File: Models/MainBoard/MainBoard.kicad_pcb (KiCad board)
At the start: 4 copper layers, 82 parts, among them J1 Conn_Coaxial, J10 Conn_01x03_Pin, J11 Conn_01x03_Pin, J12 Conn_01x03_Pin, J13 Conn_01x02_Pin, J14 Conn_01x13_Pin, J15 Conn_01x13_Pin, J16 Conn_01x24_Socket, J19 Conn_01x24_Socket, J2 Conn_Coaxial, J3 Conn_Coaxial, J4 Conn_Coaxial, J5 Conn_Coaxial, J6 Conn_Coaxial, J7 Conn_01x03_Pin, J8 Conn_01x03_Pin, J9 Conn_01x03_Pin, U1 ADS8699, U2 AD7745, U3 DAC81404, U4 DAC81401, U5 ISO7761DW, U6 ISO1641DW

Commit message: Save progress
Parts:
- J10, J11, J12, J7, J8, J9: footprint Connector_Custom:PinConnector_1x3 -> Connector_Custom:PinHeader_1x3
- J13: footprint Connector_Custom:PinConnector_1x2 -> Connector_Custom:PinHeader_1x2
- J14, J15: footprint Connector_Custom:PinConnector_1x13 -> Connector_Custom:PinHeader_1x13
- J16, J19: footprint Connector_Custom:PinConnector_1x24 -> Connector_Custom:PinSocket_1x24
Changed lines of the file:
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@@
 		(embedded_fonts no)
 	)
-	(footprint "Connector_Custom:PinConnector_1x3"
+	(footprint "Connector_Custom:PinHeader_1x3"
 		(layer "F.Cu")
 		(at 111.86 94.16)
@@
 		)
 		(embedded_fonts no)
+		(model "${KICAD9_3DMODEL_DIR}/Connector_PinHeader_2.54mm.3dshapes/PinHeader_1x03_P2.54mm_Vertical.step"
+			(offset
+				(xyz 0 2.54 0)
+			)
+			(scale
+				(xyz 1 1 1)
+			)
+			(rotate
+				(xyz -0 -0 -0)
+			)
+		)
 	)
 	(footprint "TwoTerminal:CAPC0805"
@@
 		(embedded_fonts no)
 	)
-	(footprint "Connector_Custom:PinConnector_1x3"
+	(footprint "Connector_Custom:PinHeader_1x3"
 		(layer "F.Cu")
 		(at 111.86 114.48)
@@
 		)
 		(embedded_fonts no)
+		(model "${KICAD9_3DMODEL_DIR}/Connector_PinHeader_2.54mm.3dshapes/PinHeader_1x03_P2.54mm_Vertical.step"
+			(offset
+				(xyz 0 2.54 0)
+			)
+			(scale
+				(xyz 1 1 1)
+			)
+			(rotate
+				(xyz -0 -0 -0)
+			)
+		)
 	)
 	(footprint "TwoTerminal:CAPC0603"
@@
 		)
 		(embedded_fonts no)
+		(model "${KIPRJMOD}/../libraries/IC.pretty/VQFN-32.step"
+			(offset
+				(xyz 0 0 0)
+			)
+			(scale
+				(xyz 1 1 1)
+			)
+			(rotate
+				(xyz -0 -0 -0)
+			)
+		)
 	)
 	(footprint "Connector_Custom:NetTie_0.2mm"
@@
 		(embedded_fonts no)
 	)
-	(footprint "Connector_Custom:PinConnector_1x24"
+	(footprint "Connector_Custom:PinSocket_1x24"
 		(layer "F.Cu")
 		(at 160.12 100.51)
@@
 		)
 		(embedded_fonts no)
+		(model "${KICAD9_3DMODEL_DIR}/Connector_PinSocket_2.54mm.3dshapes/PinSocket_1x24_P2.54mm_Vertical.step"
+			(offset
+				(xyz 0 29.21 0)
+			)
+			(scale
+				(xyz 1 1 1)
+			)
+			(rotate
+				(xyz -0 -0 -0)
+			)
+		)
 	)
 	(footprint "Connector_Custom:NetTie_0.2mm"
@@
 		(embedded_fonts no)
 	)
-	(footprint "Connector_Custom:PinConnector_1x24"
+	(footprint "Connector_Custom:PinSocket_1x24"
 		(layer "F.Cu")
 		(at 175.36 100.51 180)
@@
 		)
 		(embedded_fonts no)
+		(model "${KICAD9_3DMODEL_DIR}/Connector_PinSocket_2.54mm.3dshapes/PinSocket_1x24_P2.54mm_Vertical.step"
+			(offset
+				(xyz 0 29.21 0)
+			)
+			(scale
+				(xyz 1 1 1)
+			)
+			(rotate
+				(xyz -0 -0 -0)
+			)
+		)
 	)
-	(footprint "Connector_Custom:PinConnector_1x3"
+	(footprint "Connector_Custom:PinHeader_1x3"
 		(layer "F.Cu")
 		(at 111.86 124.64)
@@
 		)
 		(embedded_fonts no)
+		(model "${KICAD9_3DMODEL_DIR}/Connector_PinHeader_2.54mm.3dshapes/PinHeader_1x03_P2.54mm_Vertical.step"
+			(offset
+				(xyz 0 2.54 0)
+			)
+			(scale
+				(xyz 1 1 1)
+			)
+			(rotate
+				(xyz -0 -0 -0)
+			)
+		)
 	)
 	(footprint "TwoTerminal:CAPC0603"
@@
 		(embedded_fonts no)
 	)
-	(footprint "Connector_Custom:PinConnector_1x2"
+	(footprint "Connector_Custom:PinHeader_1x2"
 		(layer "F.Cu")
 		(at 105.51 129.72 90)
@@
 		)
 		(embedded_fonts no)
+		(model "${KICAD9_3DMODEL_DIR}/Connector_PinHeader_2.54mm.3dshapes/PinHeader_1x02_P2.54mm_Vertical.step"
+			(offset
+				(xyz 0 1.27 0)
+			)
+			(scale
+				(xyz 1 1 1)
+			)
+			(rotate
+				(xyz -0 -0 -0)
+			)
+		)
 	)
 	(footprint "TwoTerminal:CAPC0805"
@@
 		)
 		(embedded_fonts no)
+		(model "${KIPRJMOD}/../libraries/Connector_Custom.pretty/Keystone_24929.step"
+			(offset
+				(xyz 0 0 -1.5)
+			)
+			(scale
+				(xyz 1 1 1)
+			)
+			(rotate
+				(xyz -90 -0 -0)
+			)
+		)
 	)
 	(footprint "Connector_Custom:NetTie_0.2mm"
@@
 		(embedded_fonts no)
 	)
-	(footprint "Connector_Custom:PinConnector_1x3"
+	(footprint "Connector_Custom:PinHeader_1x3"
 		(layer "F.Cu")
 		(at 111.86 73.84)
@@
 		)
 		(embedded_fonts no)
+		(model "${KICAD9_3DMODEL_DIR}/Connector_PinHeader_2.54mm.3dshapes/PinHeader_1x03_P2.54mm_Vertical.step"
+			(offset
+				(xyz 0 2.54 0)
+			)
+			(scale
+				(xyz 1 1 1)
+			)
+			(rotate
+				(xyz -0 -0 -0)
+			)
+		)
 	)
 	(footprint "TwoTerminal:CAPC0603"
@@
 		(embedded_fonts no)
 	)
-	(footprint "Connector_Custom:PinConnector_1x3"
+	(footprint "Connector_Custom:PinHeader_1x3"
 		(layer "F.Cu")
 		(at 111.86 104.32)
@@
 		)
 		(embedded_fonts no)
+		(model "${KICAD9_3DMODEL_DIR}/Connector_PinHeader_2.54mm.3dshapes/PinHeader_1x03_P2.54mm_Vertical.step"
+			(offset
+				(xyz 0 2.54 0)
+			)
+			(scale
+				(xyz 1 1 1)
+			)
+			(rotate
+				(xyz -0 -0 -0)
+			)
+		)
 	)
 	(footprint "TwoTerminal:CAPC0805"
@@
 		(embedded_fonts no)
 	)
-	(footprint "Connector_Custom:PinConnector_1x3"
+	(footprint "Connector_Custom:PinHeader_1x3"
 		(layer "F.Cu")
 		(at 111.86 84)
@@
 		)
 		(embedded_fonts no)
+		(model "${KICAD9_3DMODEL_DIR}/Connector_PinHeader_2.54mm.3dshapes/PinHeader_1x03_P2.54mm_Vertical.step"
+			(offset
+				(xyz 0 2.54 0)
+			)
+			(scale
+				(xyz 1 1 1)
+			)
+			(rotate
+				(xyz -0 -0 -0)
+			)
+		)
 	)
 	(footprint "TwoTerminal:CAPC0603"
@@
 		)
 		(embedded_fonts no)
+		(model "${KIPRJMOD}/../libraries/Connector_Custom.pretty/Molex_MCX.step"
+			(offset
+				(xyz -6.53 0 3.3)
+			)
+			(scale
+				(xyz 1 1 1)
+			)
+			(rotate
+				(xyz -90 -0 90)
+			)
+		)
 	)
 	(footprint "TwoTerminal:RESC0603"
@@
 		)
 		(embedded_fonts no)
+		(model "${KIPRJMOD}/../libraries/Connector_Custom.pretty/Molex_MCX.step"
+			(offset
+				(xyz -6.53 0 3.3)
+			)
+			(scale
+				(xyz 1 1 1)
+			)
+			(rotate
+				(xyz -90 -0 90)
+			)
+		)
 	)
 	(footprint "Connector_Custom:Molex_MCX"
@@
 		)
 		(embedded_fonts no)
+		(model "${KIPRJMOD}/../libraries/Connector_Custom.pretty/Molex_MCX.step"
+			(offset
+				(xyz -6.53 0 3.3)
+			)
+			(scale
+				(xyz 1 1 1)
+			)
+			(rotate
+				(xyz -90 -0 90)
+			)
+		)
 	)
 	(footprint "TwoTerminal:RESC0603"
@@
 		(embedded_fonts no)
 	)
-	(footprint "Connector_Custom:PinConnector_1x13"
+	(footprint "Connector_Custom:PinHeader_1x13"
 		(layer "B.Cu")
 		(at 132.18 71.3 -90)
@@
 		)
 		(property "Purchase Link" "https://www.digikey.com/en/products/detail/sullins-connector-solutions/PRPC024SAAN-RC/2775230"
-			(at 0 0 90)
+			(at 0 0 270)
 			(unlocked yes)
 			(layer "B.Fab")
@@
 		)
 		(property "Cost" "$0.563"
-			(at 0 0 90)
+			(at 0 0 270)
 			(unlocked yes)
 			(layer "B.Fab")
@@
 		)
 		(embedded_fonts no)
+		(model "${KICAD9_3DMODEL_DIR}/Connector_PinHeader_2.54mm.3dshapes/PinHeader_1x13_P2.54mm_Vertical.step"
+			(offset
+				(xyz 0 15.24 0)
+			)
+			(scale
+				(xyz 1 1 1)
+			)
+			(rotate
+				(xyz -0 -0 -0)
+			)
+		)
 	)
 	(footprint "TwoTerminal:RESC0603"
@@
 		(embedded_fonts no)
 	)
-	(footprint "Connector_Custom:PinConnector_1x13"
+	(footprint "Connector_Custom:PinHeader_1x13"
 		(layer "B.Cu")
 		(at 132.18 129.72 -90)
@@
 		)
 		(embedded_fonts no)
+		(model "${KICAD9_3DMODEL_DIR}/Connector_PinHeader_2.54mm.3dshapes/PinHeader_1x13_P2.54mm_Vertical.step"
+			(offset
+				(xyz 0 15.24 0)
+			)
+			(scale
+				(xyz 1 1 1)
+			)
+			(rotate
+				(xyz -0 -0 -0)
+			)
+		)
 	)
 	(footprint "Connector_Custom:Molex_MCX"
@@
 		)
 		(embedded_fonts no)
+		(model "${KIPRJMOD}/../libraries/Connector_Custom.pretty/Molex_MCX.step"
+			(offset
+				(xyz -6.53 0 3.3)
+			)
+			(scale
+				(xyz 1 1 1)
+			)
+			(rotate
+				(xyz -90 -0 90)
+			)
+		)
 	)
 	(footprint "TwoTerminal:RESC0603"
@@
 		)
 		(embedded_fonts no)
+		(model "${KIPRJMOD}/../libraries/Connector_Custom.pretty/Molex_MCX.step"
+			(offset
+				(xyz -6.53 0 3.3)
+			)
+			(scale
+				(xyz 1 1 1)
+			)
+			(rotate
+				(xyz -90 -0 90)
+			)
+		)
 	)
 	(footprint "Connector_Custom:Molex_MCX"
@@
 		)
 		(embedded_fonts no)
+		(model "${KIPRJMOD}/../libraries/Connector_Custom.pretty/Molex_MCX.step"
+			(offset
+				(xyz -6.53 0 3.3)
+			)
+			(scale
+				(xyz 1 1 1)
+			)
+			(rotate
+				(xyz -90 -0 90)
+			)
+		)
 	)
 	(gr_text "Nanofactory Project\nPhase 0.2/I/II"

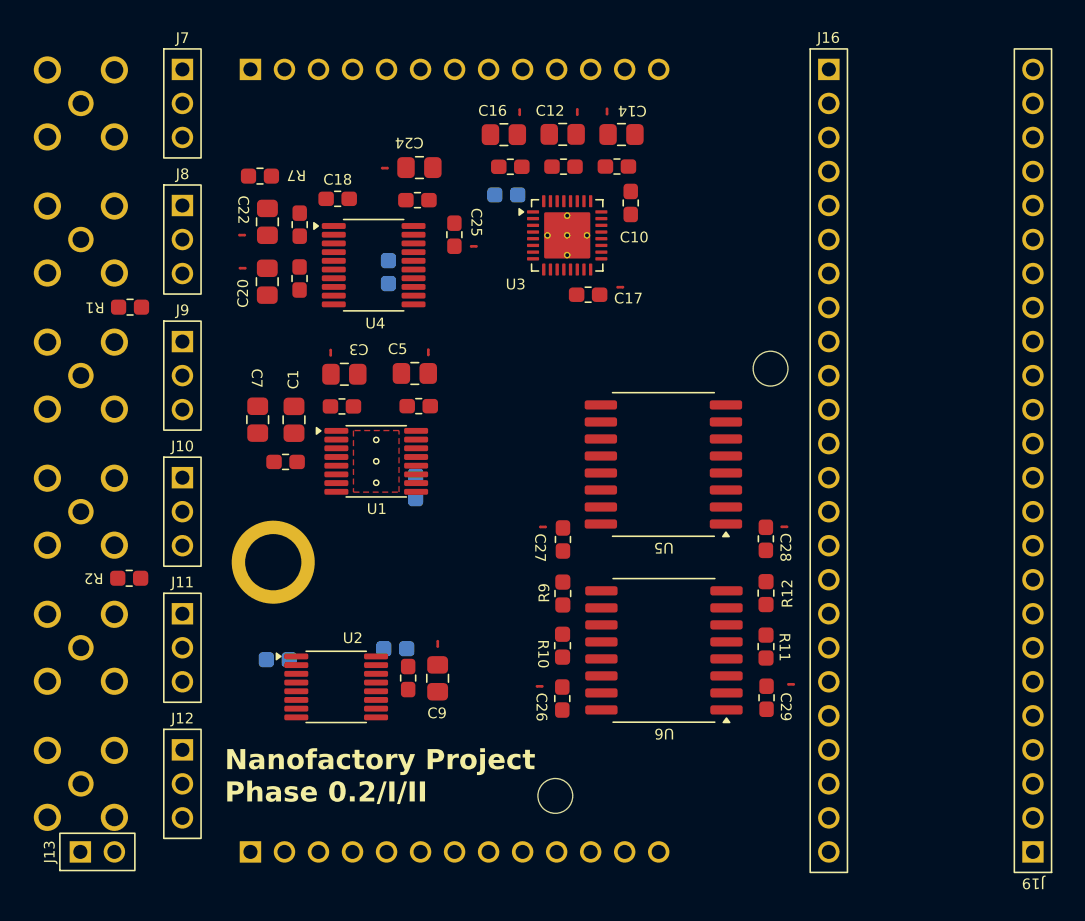
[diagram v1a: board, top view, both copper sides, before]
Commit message: Save progress
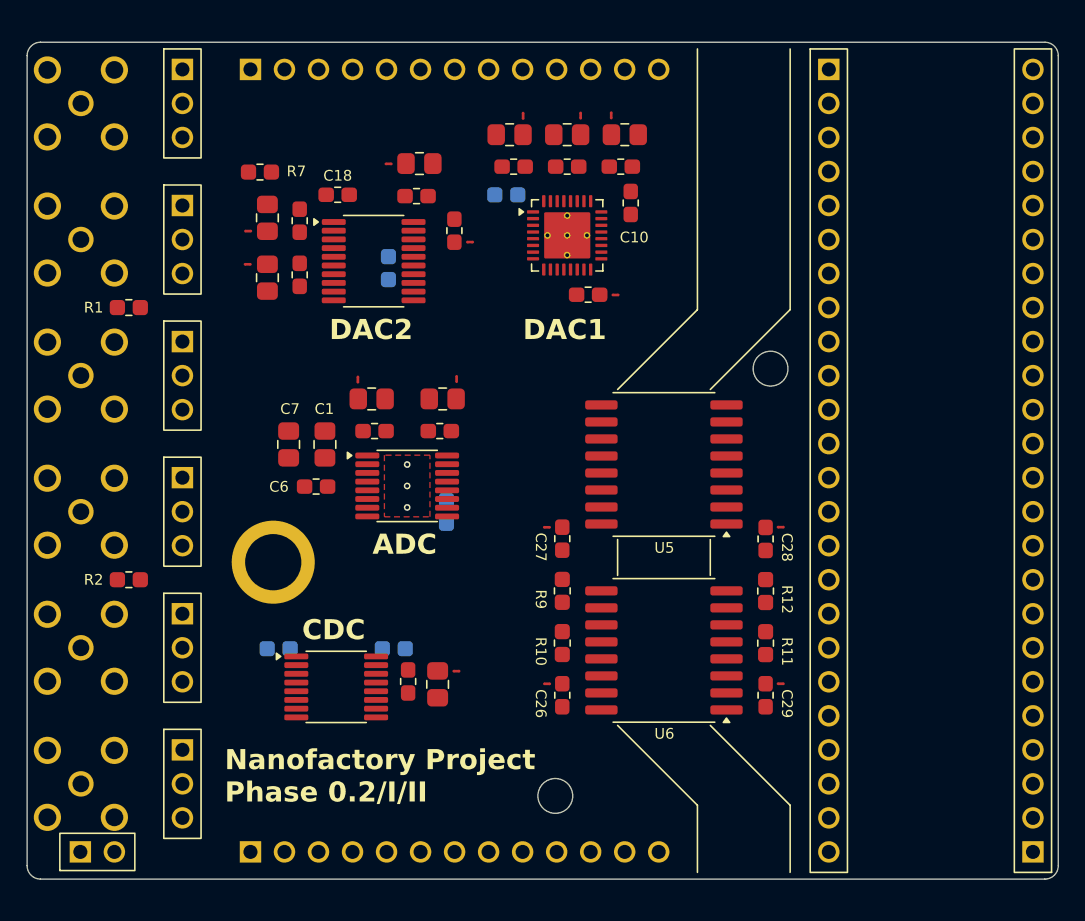
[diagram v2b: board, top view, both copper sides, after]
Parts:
- moved C2 3.05 mm to (126.2, 98.3)
- moved C7 2.96 mm to (119.8, 99.3)
- moved C1 2.95 mm to (122.5, 99.3)
- moved U1 2.95 mm to (128.6, 102.4)
- moved R3 2.94 mm to (131.6, 104.3)
- moved C6 2.93 mm to (121.8, 102.4)
- moved NT2 2.90 mm to (132.3, 94.4)
- moved NT1 2.85 mm to (125.0, 94.5)
- moved C5 2.82 mm to (131.3, 95.9)
- moved C3 2.75 mm to (126.0, 95.9)
- moved NT3 2.47 mm to (132.3, 116.2), turned to 0 degrees
- moved C4 2.44 mm to (131.1, 98.3)
- moved R4 0.82 mm to (119.0, 114.5)
- moved NT15 0.77 mm to (156.5, 117.2)
- moved NT7 0.68 mm to (144.2, 88.1)
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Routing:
- added copper zone on In1.Cu, net /Isolation/GND_Digital
- added copper zone on In1.Cu, net GND
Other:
- board outline added: 77 x 62.5 mm
- board text added: "ADC"
- board text added: "CDC"
- board text added: "DAC1"
- board text added: "DAC2"
